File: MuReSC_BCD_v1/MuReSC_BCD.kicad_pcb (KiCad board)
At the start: 4 copper layers, 75 parts, among them J1 Conn_Coaxial:60312002114503, J10 Conn_Coaxial:60312002114503, J11 Conn_Coaxial:60312002114503, J12 Conn_Coaxial:60312002114503, J13 Conn_Coaxial:60312002114503, J2 Conn_Coaxial:60312002114503, J3 Conn_Coaxial:60312002114503, J4 Conn_Coaxial:60312002114503, J5 Conn_Coaxial:60312002114503, J6 Conn_01x04_Socket, J7 Conn_Coaxial:60312002114503, J8 Conn_Coaxial:60312002114503, J9 Conn_Coaxial:60312002114503, SW1 SW_DIP_x05, SW2 SW_DIP_x05, SW3 SW_DIP_x05

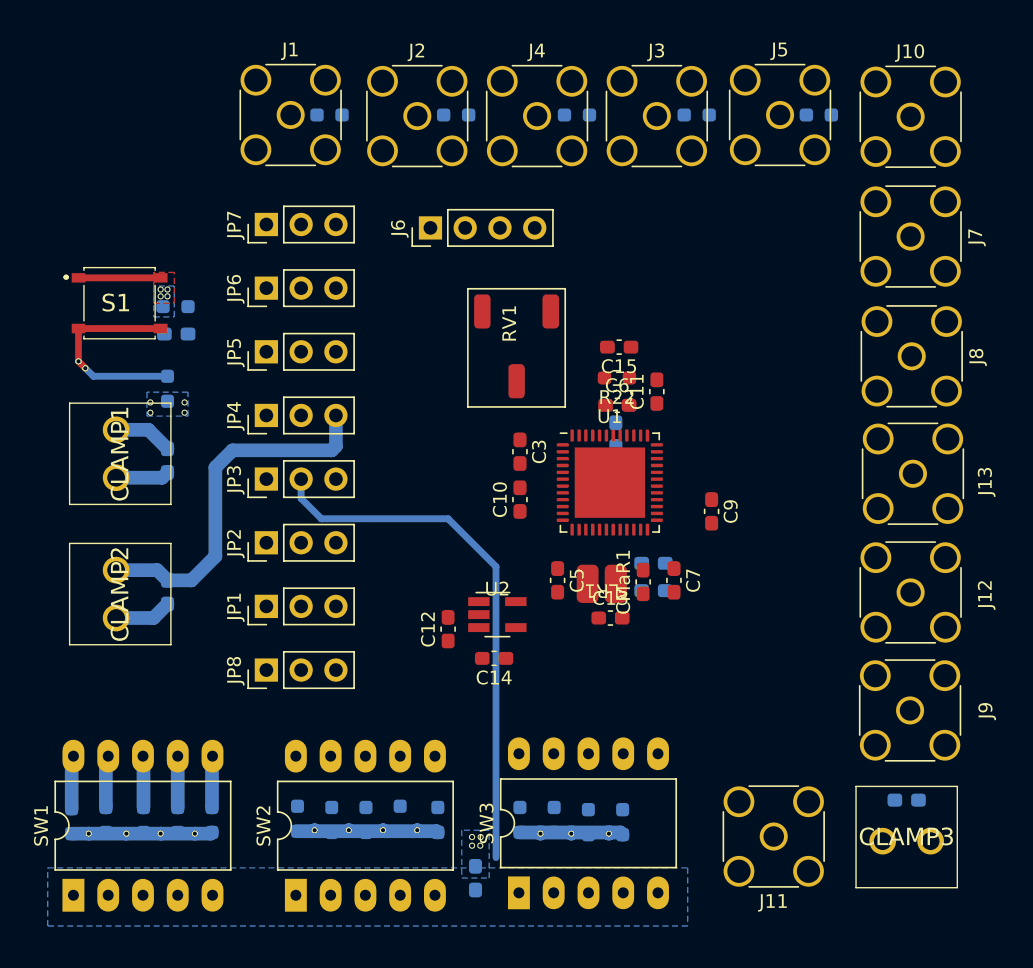
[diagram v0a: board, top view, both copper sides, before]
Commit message: up
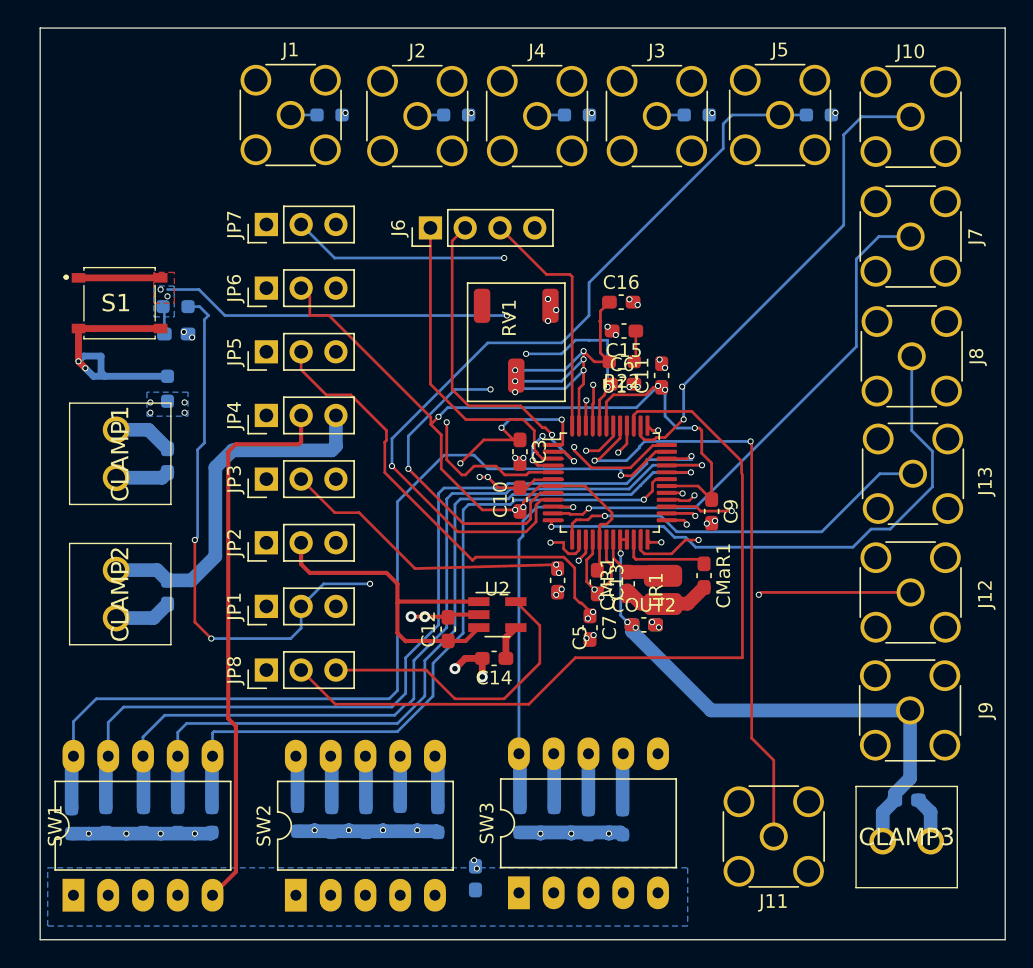
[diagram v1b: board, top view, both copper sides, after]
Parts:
- C16, CMR1, COUT2: moved to F.Cu
- U1: footprint Package_DFN_QFN:QFN-48-1EP_7x7mm_P0.5mm_EP5.15x5.15mm -> Package_QFP:TQFP-48_7x7mm_P0.5mm
- moved C16 9.69 mm to (109.2, 86.4), turned to 0 degrees
- moved C7 7.04 mm to (106.9, 110.2)
- moved COUT1 4.55 mm to (110.8, 110.0)
- moved LR1 4.50 mm to (112.2, 107.4), turned to 90 degrees
- moved CMaR1 4.47 mm to (115.2, 106.4), turned to -90 degrees
- moved C13 2.79 mm to (107.4, 106.9), turned to -90 degrees
- moved COUT2 2.60 mm to (110.8, 110.0)
- moved CMR1 1.95 mm to (109.6, 107.0), turned to 90 degrees
- moved C6 1.58 mm to (109.2, 92.4)
- moved C11 1.23 mm to (112.1, 91.8)
- moved C15 1.23 mm to (109.3, 88.5)
- moved R22 1.23 mm to (109.2, 90.8)
- moved RV1 0.41 mm to (101.5, 88.6)
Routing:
- net /VDD_IO: track 0.00 -> 79.5 mm, vias 0 -> 6
- net /VBATT: track 0.00 -> 65.3 mm, vias 0 -> 6
- net /DT_D0: track 3.89 -> 67.7 mm, vias 0 -> 1
- net /DT_D1: track 3.82 -> 66.4 mm, vias 0 -> 1
- net /DRIVE_G4: track 0.00 -> 60.7 mm, vias 0 -> 1
- net /DT_D2: track 3.76 -> 64.1 mm, vias 0 -> 1
- net /V1V8O: track 0.00 -> 59.3 mm
- net /SEL_OPEN_LOOP: track 0.00 -> 57.6 mm, vias 0 -> 1
- net /SEL_INT_REF: track 0.00 -> 57.4 mm, vias 0 -> 1
- net /DRIVE_G3: track 0.00 -> 56.9 mm, vias 0 -> 2
- net /DT_D3: track 3.75 -> 59.6 mm, vias 0 -> 1
- net /SEL_CLK: track 0.00 -> 53.7 mm, vias 0 -> 1
- net /ADT_D1: track 0.00 -> 51.9 mm, vias 0 -> 1
- net /ADT_D4: track 0.00 -> 51.4 mm, vias 0 -> 1
- net /EXT_CLK: track 0.00 -> 50.6 mm, vias 0 -> 1
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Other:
- board outline added: 70.5 x 66.6 mm
